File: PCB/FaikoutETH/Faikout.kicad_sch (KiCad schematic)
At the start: 71 parts, among them J1 1x5, J2 TC2030-USB-NL, J3 Reset, J4 RJ45_LED, Q1 BSS138PS, U2 KSZ8851SNL, U4 ESP32-S3-MINI-1, U5 TPS62933, Y1 Crystal_GND24

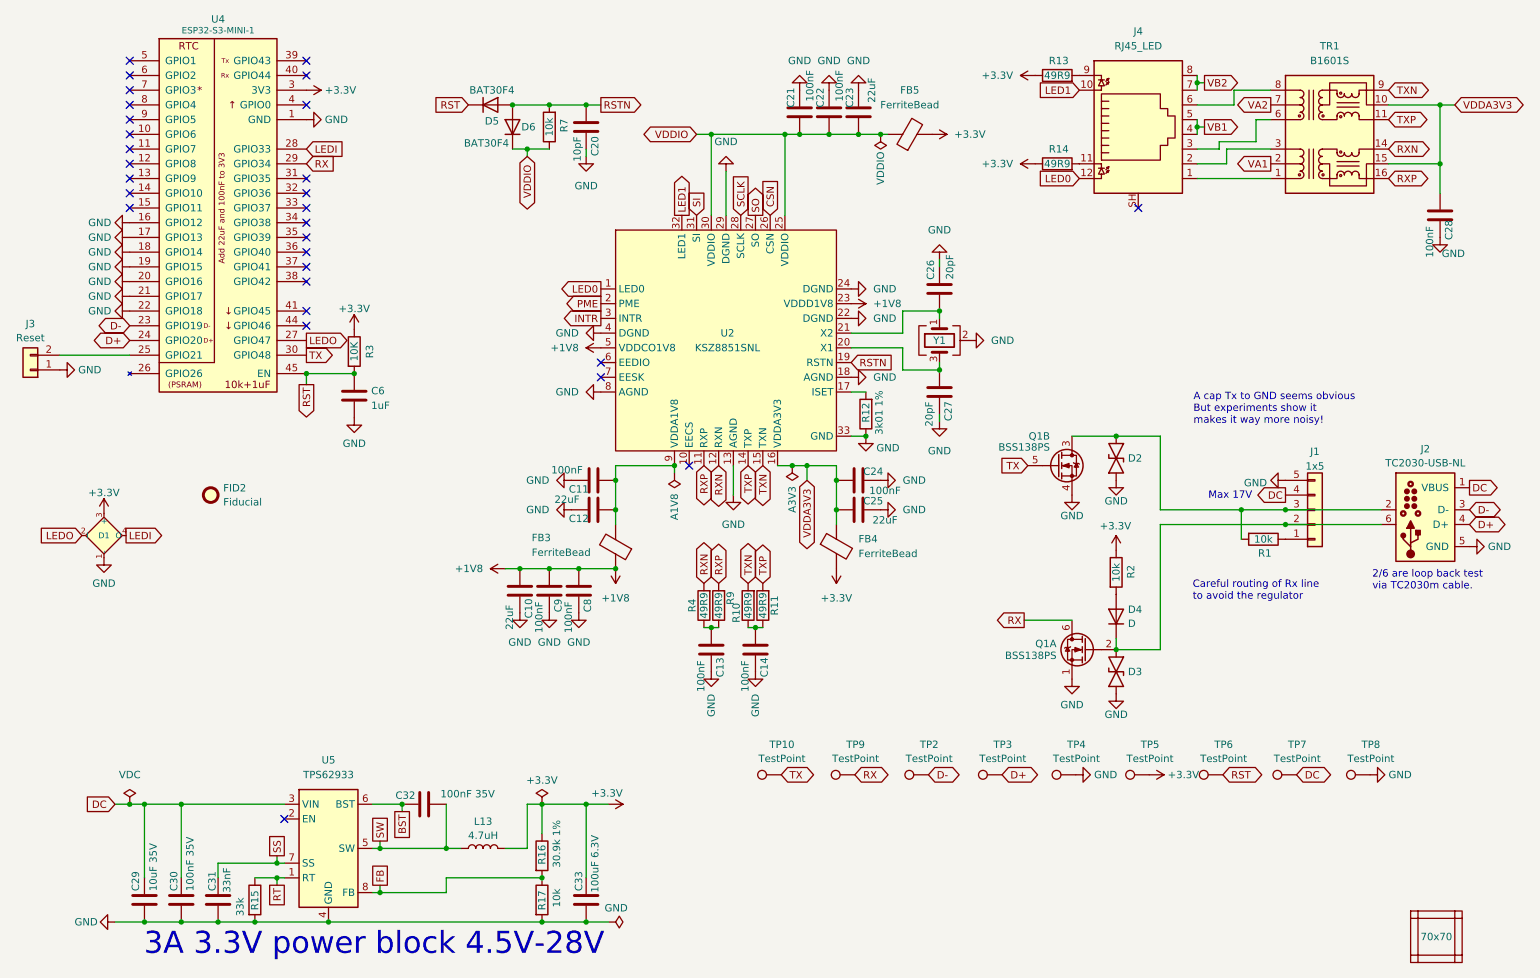
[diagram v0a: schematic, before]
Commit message: Ethernet board
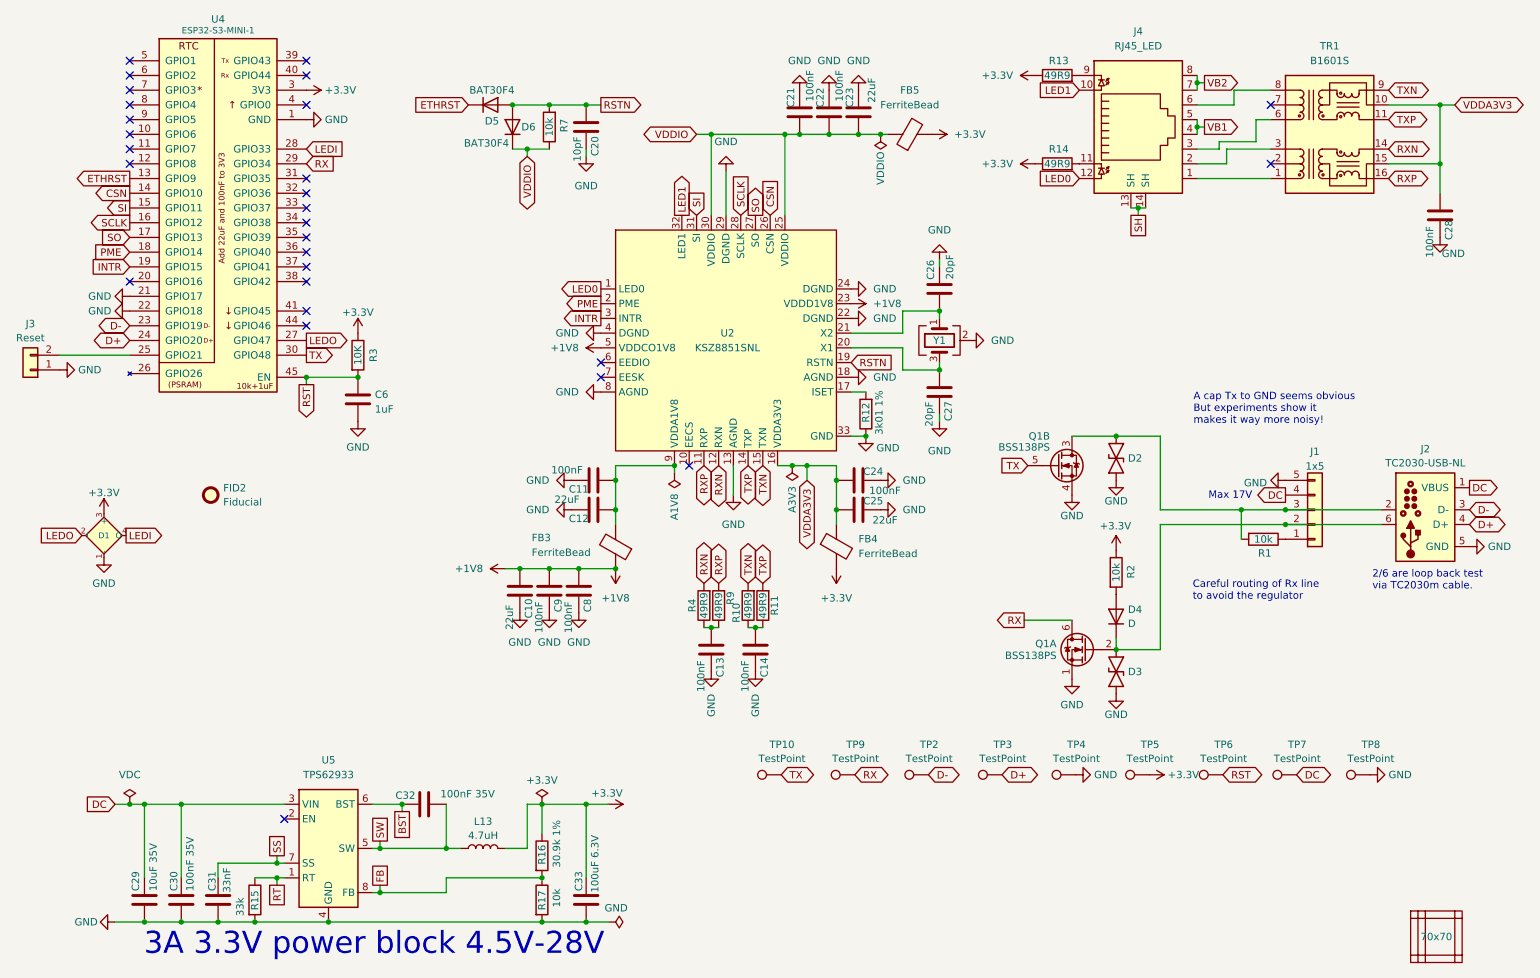
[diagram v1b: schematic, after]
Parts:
- added V7: (no value), RevK:VCUT70N, symbol RevK:VCUT
- U2: footprint Package_DFN_QFN:QFN-32-1EP_5x5mm_P0.5mm_EP3.7x3.7mm -> RevK:QFN-32-1EP_5x5mm_P0.5mm_EP3.7x3.7mm
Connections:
- net CSN: now also U4.14 (GPIO10)
- net GND: no longer U4.16 (GPIO12), U4.17 (GPIO13), U4.18 (GPIO14), U4.19 (GPIO15), U4.20 (GPIO16)
- net INTR: now also U4.19 (GPIO15)
- net PME: now also U4.18 (GPIO14)
- net RST: no longer D5.1 (K)
- net SCLK: now also U4.16 (GPIO12)
- net SI: now also U4.15 (GPIO11)
- net SO: now also U4.17 (GPIO13)
- net ETHRST: now reaches U4.13 (GPIO9)
- net ETHRST: now also D5.1 (K)
- net VA1: no longer names the net of TR1.2 (C_TD)
- net VA2: no longer names the net of TR1.7 (C_RD)
- new net SH: J4.13 (SH), J4.14 (SH)
- no-connect marks 29 -> 28
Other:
- moved on the sheet: C6, R3

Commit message: Library update
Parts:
- FB3, FB4, FB5: footprint Inductor_SMD:L_0603_1608Metric -> RevK:L_0603
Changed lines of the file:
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@@
 			)
 		)
-		(property "Footprint" "Inductor_SMD:L_0603_1608Metric"
+		(property "Footprint" "RevK:L_0603"
 			(at 156.972 106.68 90)
 			(hide yes)
@@
 			)
 		)
-		(property "Footprint" "Inductor_SMD:L_0603_1608Metric"
+		(property "Footprint" "RevK:L_0603"
 			(at 122.428 106.68 90)
 			(hide yes)
@@
 			)
 		)
-		(property "Footprint" "Inductor_SMD:L_0603_1608Metric"
+		(property "Footprint" "RevK:L_0603"
 			(at 171.45 37.338 90)
 			(hide yes)
